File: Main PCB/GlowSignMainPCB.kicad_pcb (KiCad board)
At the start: 2 copper layers, 169.5 x 83.5 mm, 130 parts, among them P1 Solder_Pad, P2 Solder_Pad, SW1 TS-1185EC-C-D-B, SW2 TS-1185EC-C-D-B, SW3 TS24CA, U12 AO3400A, U13 AP40P05, U14 AP40P05, U16 AP40P05, U17 SS54, U18 BL1117-33CX, U19 TPS3839G33DBZR, U2 SS54, U20 MSM261D4030H1CPM, U3 SN74LVC2T45DCUR, U4 ESP32-WROOM-32E, U7 CP2102-GMR, U8 UMH3N

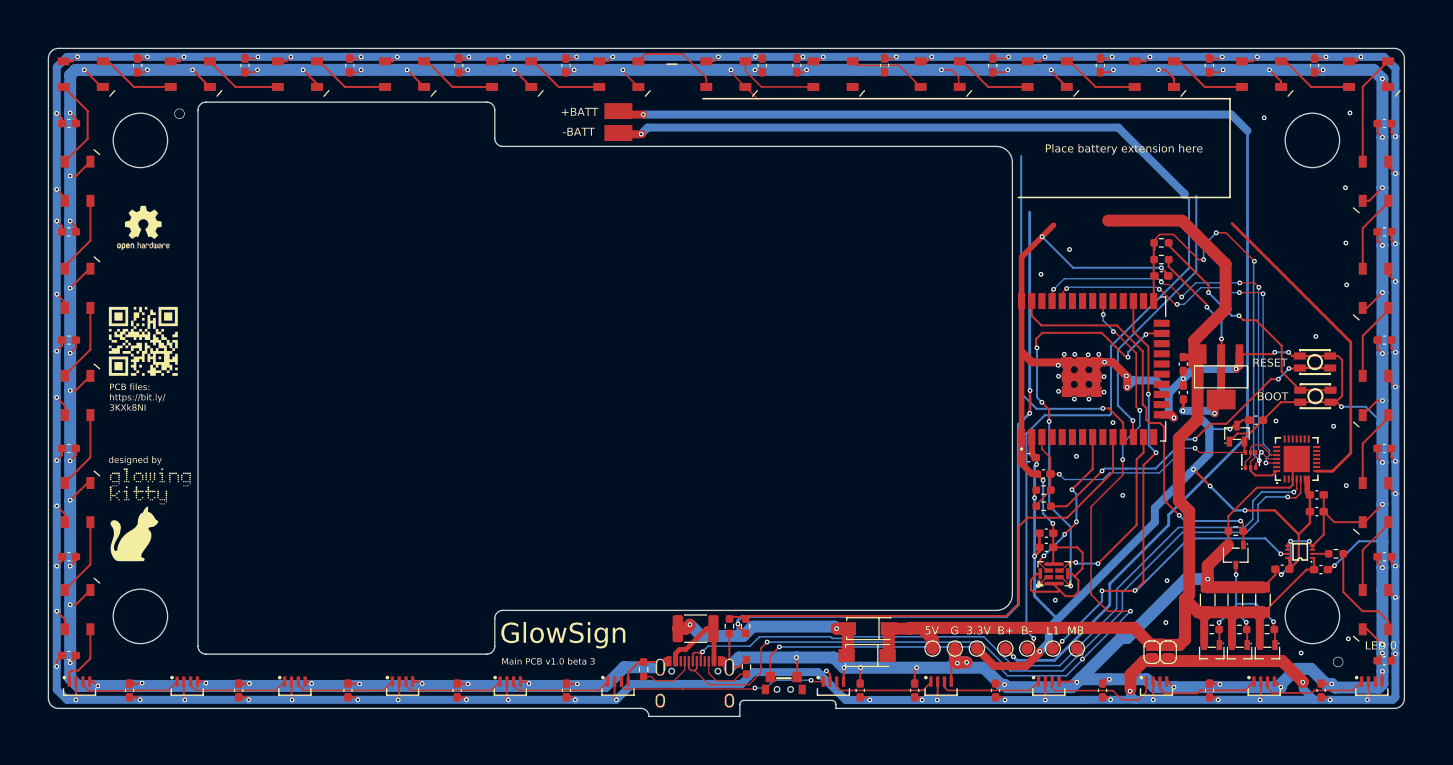
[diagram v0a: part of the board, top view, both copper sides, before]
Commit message: updated pcb files
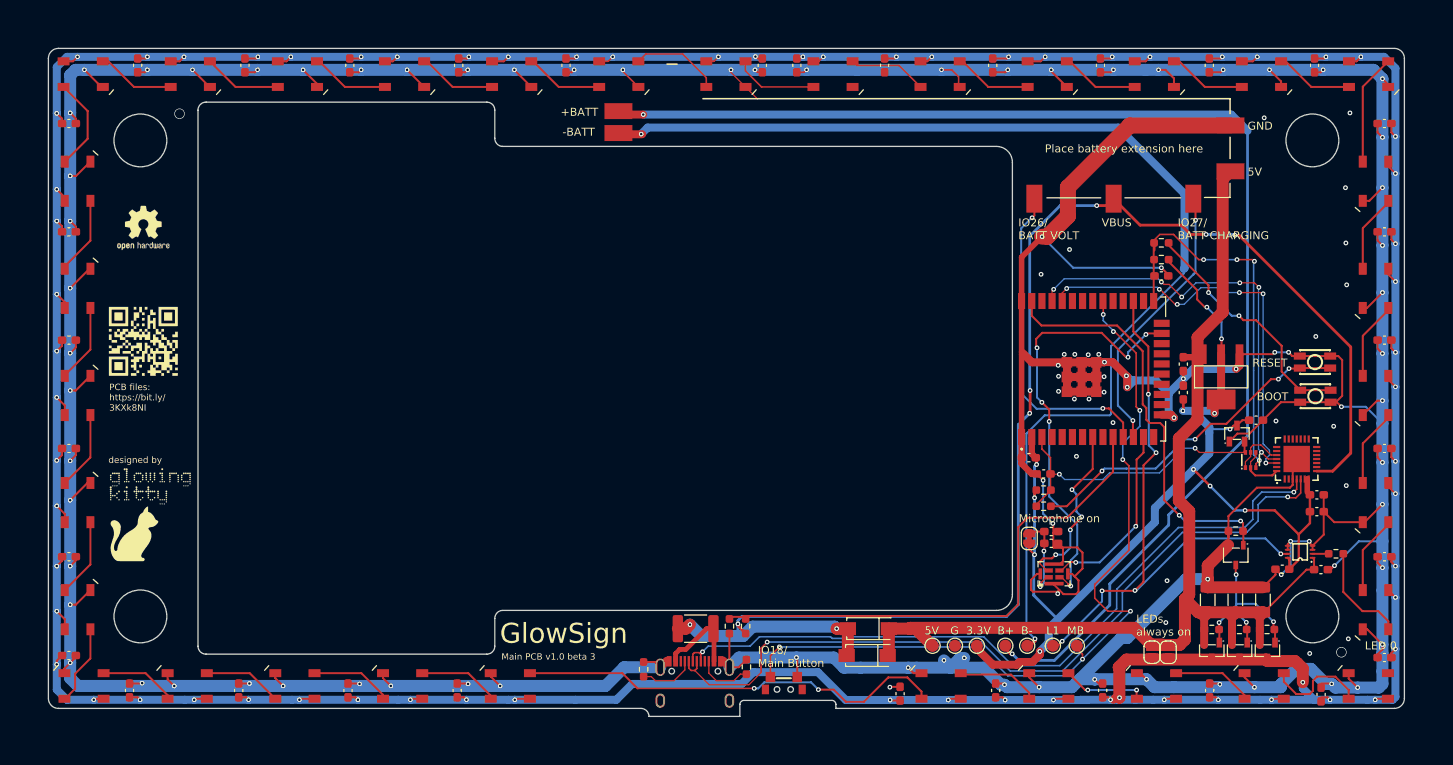
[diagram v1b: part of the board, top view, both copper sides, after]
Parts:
- removed the C46 at (131.2, 139.6)
- removed the C47 at (167.9, 139.6)
- removed the D31 at (137.6, 139.3)
- removed the D32 at (164.5, 139.3)
- added JP3: SolderJumper_2_Bridged, Jumper:SolderJumper-2_P1.3mm_Bridged_RoundedPad1.0x1.5mm, F.Cu at (189.0, 120.6)
- added P3: Solder_Pad, footprint:Solder pad, F.Cu at (189.7, 78.1)
- added P4: Solder_Pad, footprint:Solder pad, F.Cu at (199.6, 78.1)
- added P5: Solder_Pad, footprint:Solder pad, F.Cu at (209.6, 78.1)
- added P6: Solder_Pad, footprint:Solder pad, F.Cu at (214.1, 74.6)
- added P7: Solder_Pad, footprint:Solder pad, F.Cu at (214.1, 68.9)
- D26, D27, D28, D29, D30: value WS2812B-4020 -> WS2812B; footprint footprint:LED-SMD_WS2812B-4020 -> LED_SMD:LED_WS2812B_PLCC4_5.0x5.0mm_P3.2mm
- D31: renamed from D33; value WS2812B-4020 -> WS2812B; footprint footprint:LED-SMD_WS2812B-4020 -> LED_SMD:LED_WS2812B_PLCC4_5.0x5.0mm_P3.2mm
- D32: renamed from D34; value WS2812B-4020 -> WS2812B; footprint footprint:LED-SMD_WS2812B-4020 -> LED_SMD:LED_WS2812B_PLCC4_5.0x5.0mm_P3.2mm
- D33: renamed from D35; value WS2812B-4020 -> WS2812B; footprint footprint:LED-SMD_WS2812B-4020 -> LED_SMD:LED_WS2812B_PLCC4_5.0x5.0mm_P3.2mm
- D34: renamed from D36; value WS2812B-4020 -> WS2812B; footprint footprint:LED-SMD_WS2812B-4020 -> LED_SMD:LED_WS2812B_PLCC4_5.0x5.0mm_P3.2mm
- D35: renamed from D37; value WS2812B-4020 -> WS2812B; footprint footprint:LED-SMD_WS2812B-4020 -> LED_SMD:LED_WS2812B_PLCC4_5.0x5.0mm_P3.2mm
- moved C46 1.87 mm to (172.9, 140.0)
- moved C10 0.79 mm to (191.8, 121.2)
- moved C53 0.64 mm to (191.8, 119.7)
- moved D26 0.64 mm to (70.9, 139.0)
- moved D35 0.55 mm to (231.4, 139.0)
- moved C50 0.51 mm to (225.5, 140.1)
- moved C18 0.41 mm to (233.4, 135.5)
- moved TP1 0.36 mm to (192.0, 134.0)
- moved TP2 0.36 mm to (195.0, 134.0)
- moved TP4 0.36 mm to (186.0, 134.0)
- moved TP5 0.36 mm to (188.8, 134.0)
- moved TP6 0.36 mm to (182.5, 134.0)
- moved TP7 0.36 mm to (179.7, 134.0)
- moved TP8 0.36 mm to (176.9, 134.0)
- moved D27 0.30 mm to (83.8, 139.0)
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- renumbered C48 to C46, C49 to C47, C50 to C48, C51 to C49, C52 to C50
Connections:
- C10 pad 2: +3V3 -> Net-(C10-Pad2)
- C53 pad 2: +3V3 -> Net-(C10-Pad2)
- D26 pad 1: Net-(D25-Pad2) -> LED 5V
- D26 pad 2: LED 5V -> Net-(D26-Pad2)
- D26 pad 3: Net-(D26-Pad3) -> GND
- D26 pad 4: GND -> Net-(D25-Pad2)
- D27 pad 1: Net-(D26-Pad3) -> LED 5V
- D27 pad 2: LED 5V -> Net-(D27-Pad2)
- D27 pad 3: Net-(D27-Pad3) -> GND
- D27 pad 4: GND -> Net-(D26-Pad2)
- D28 pad 1: Net-(D27-Pad3) -> LED 5V
- D28 pad 2: LED 5V -> Net-(D28-Pad2)
- D28 pad 3: Net-(D28-Pad3) -> GND
- D28 pad 4: GND -> Net-(D27-Pad2)
- D29 pad 1: Net-(D28-Pad3) -> LED 5V
- D29 pad 2: LED 5V -> Net-(D29-Pad2)
- D29 pad 3: Net-(D29-Pad3) -> GND
- D29 pad 4: GND -> Net-(D28-Pad2)
- D30 pad 1: Net-(D29-Pad3) -> LED 5V
- D30 pad 2: LED 5V -> Net-(D30-Pad2)
- D30 pad 3: Net-(D30-Pad3) -> GND
- D30 pad 4: GND -> Net-(D29-Pad2)
- D31 pad 1: Net-(D32-Pad3) -> LED 5V
- D31 pad 2: LED 5V -> Net-(D31-Pad2)
- D31 pad 3: Net-(D33-Pad3) -> GND
- D31 pad 4: GND -> Net-(D30-Pad2)
- D32 pad 1: Net-(D33-Pad3) -> LED 5V
- D32 pad 2: LED 5V -> Net-(D32-Pad2)
- D32 pad 3: Net-(D34-Pad3) -> GND
- D32 pad 4: GND -> Net-(D31-Pad2)
- D33 pad 1: Net-(D34-Pad3) -> LED 5V
- D33 pad 2: LED 5V -> Net-(D33-Pad2)
- D33 pad 3: Net-(D35-Pad3) -> GND
- D33 pad 4: GND -> Net-(D32-Pad2)
- D34 pad 1: Net-(D35-Pad3) -> LED 5V
- D34 pad 2: LED 5V -> Net-(D34-Pad2)
- D34 pad 3: Net-(D36-Pad3) -> GND
- D34 pad 4: GND -> Net-(D33-Pad2)
- D35 pad 1: Net-(D36-Pad3) -> LED 5V
- D35 pad 2: LED 5V -> (no net)
- D35 pad 3: unconnected-(D37-Pad3) -> GND
- D35 pad 4: GND -> Net-(D34-Pad2)
- U20 pad 1: +3V3 -> Net-(C10-Pad2)
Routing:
- net Net-(D30-Pad2): track 0.00 -> 54.4 mm, vias 0 -> 2
- net Net-(D31-Pad3): track 26.5 -> 0.00 mm, vias 2 -> 0
- net GND: track 915.7 -> 941.1 mm, vias 117 -> 112
- net VBUS: track 155.5 -> 180.6 mm, vias 5 -> 8
- net Net-(D34-Pad3): track 14.9 -> 0.00 mm
- net Net-(D35-Pad3): track 13.5 -> 0.00 mm
- net Net-(D36-Pad3): track 13.4 -> 0.00 mm
- net Net-(D34-Pad2): track 0.00 -> 13.2 mm
- net Net-(D33-Pad3): track 13.1 -> 0.00 mm
- net Net-(D32-Pad3): track 13.1 -> 0.00 mm
- net Net-(D26-Pad3): track 13.0 -> 0.00 mm
- net Net-(D29-Pad3): track 12.9 -> 0.00 mm
- net Net-(D30-Pad3): track 12.9 -> 0.00 mm
- net Net-(D28-Pad3): track 12.9 -> 0.00 mm
- net Net-(D27-Pad3): track 12.9 -> 0.00 mm
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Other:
- outline, holes or cut-outs redrawn
- board text added: "GND"
- board text added: "IO18/ Main Button"
- board text added: "IO26/ BATT VOLT"
- board text added: "IO27/ BATT CHARGING"
- board text added: "LEDs always on"
- board text added: "Microphone on"
- board text added: "VBUS"
